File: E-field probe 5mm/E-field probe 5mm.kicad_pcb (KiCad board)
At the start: 2 copper layers, 100 x 11 mm, 1 part, among them J1 Conn_Coaxial

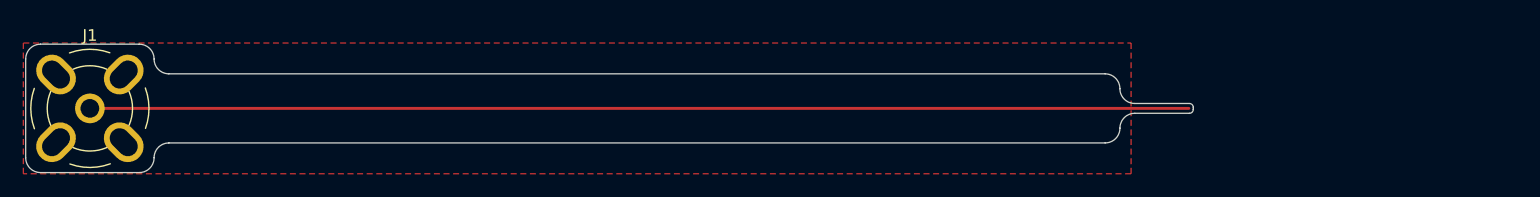
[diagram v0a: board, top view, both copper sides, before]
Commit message: initial design of all probes
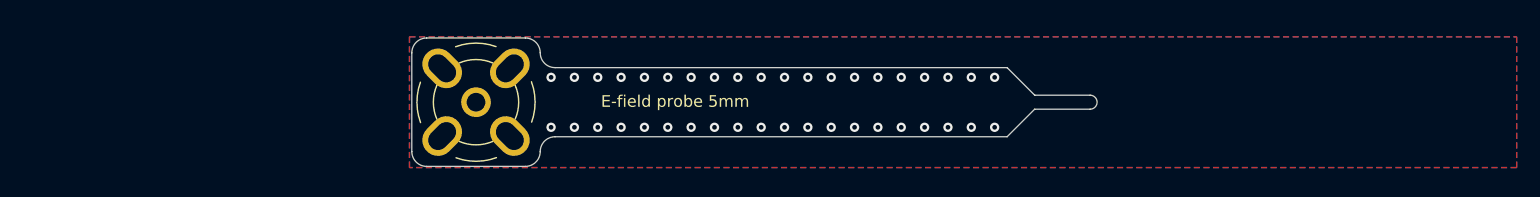
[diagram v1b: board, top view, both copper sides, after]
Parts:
- moved J1 33.1 mm to (110.9, 96.3)
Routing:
- net Net-(J1-Pad1): track 94.1 -> 52.8 mm
- net GND: vias 0 -> 40
- added copper zone on B.Cu, net GND
- added copper zone on In2.Cu, net GND
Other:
- board size 100 x 11 mm -> 58.7 x 11 mm
- copper layers 2 -> 4
- net class Default: clearance 0.2 -> 0.1; trace_width 0.25 -> 0.706149
- rule trace_clearance: 0.2 -> 0.1
- board text added: "E-field probe 5mm"
- board text removed: "todo: via fence outline shape"
